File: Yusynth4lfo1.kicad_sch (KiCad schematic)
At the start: 40 parts, among them J1 Conn_01x13_Male, J3 Conn_02x05_Counter_Clockwise, Q2 BC557C, Q3 BC557C, U1 LM13700, U2 TL074, U3 TL074

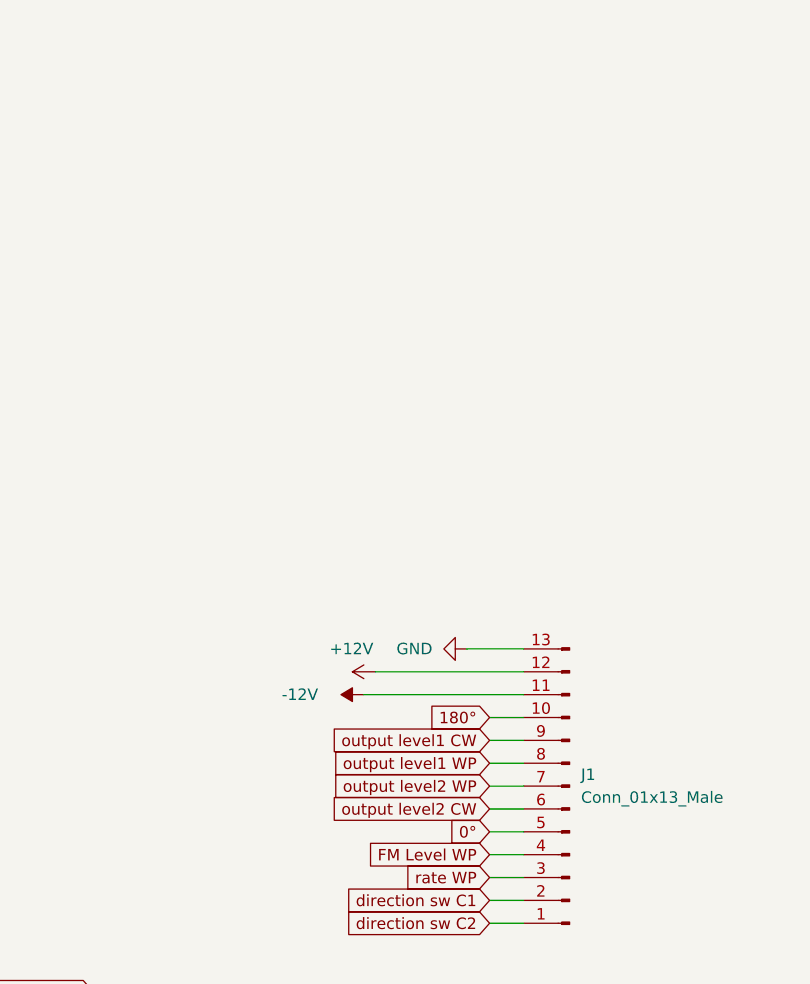
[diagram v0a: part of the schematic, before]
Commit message: derniere version vérifié
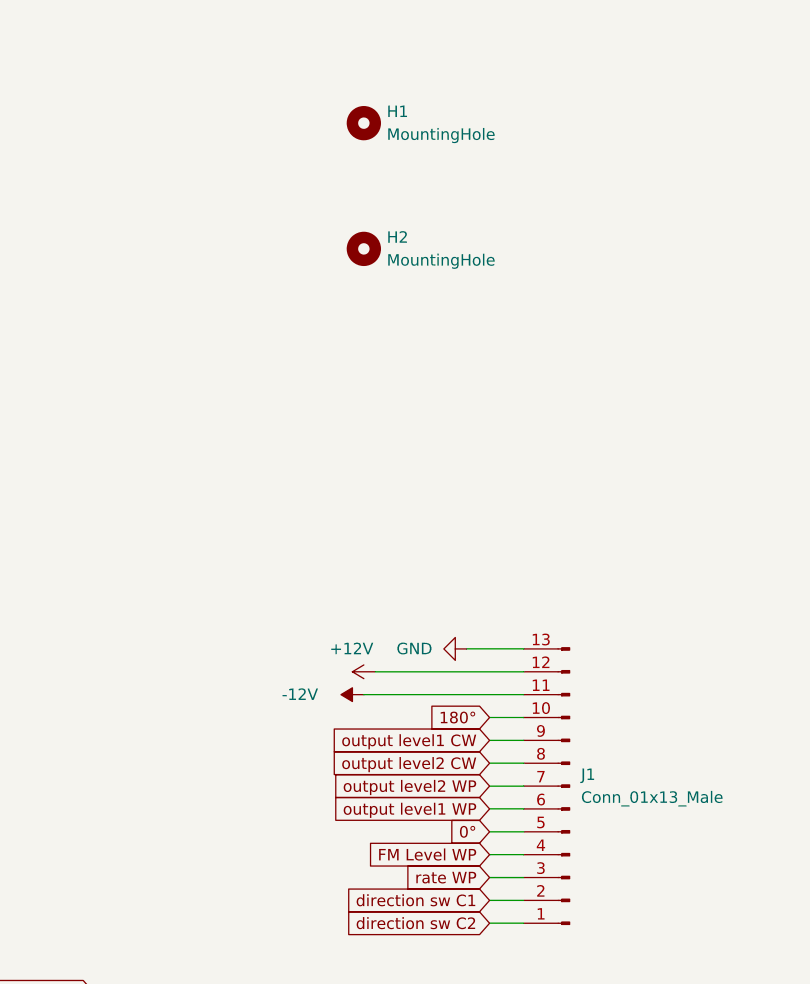
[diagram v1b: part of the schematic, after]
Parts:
- added H1, H2: MountingHole, MountingHole:MountingHole_3.2mm_M3, symbol Mechanical:MountingHole
- Q2, Q3: footprint Package_TO_SOT_THT:TO-92_Inline -> Package_TO_SOT_THT:TO-92_HandSolder
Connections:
- net output level1 WP: now also J1.6 (Pin_6); no longer J1.8 (Pin_8)
- net output level2 CW: now also J1.8 (Pin_8); no longer J1.6 (Pin_6)
